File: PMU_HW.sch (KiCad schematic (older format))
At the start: 9 parts, among them J1 Conn_01x08_Male, J2 Conn_01x08_Male, J3 Conn_01x02_Female, U2 ADS8681IPWR

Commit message: lul
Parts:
- U2: symbol Analog_ADC:ADS8681IPWR -> Analog_ADC:ADS8681IRPWR
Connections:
- wire segments 22 -> 35
- no-connect marks 0 -> 3
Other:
- moved on the sheet: C1, C2, C3, C4, C5, J1, J2, J3

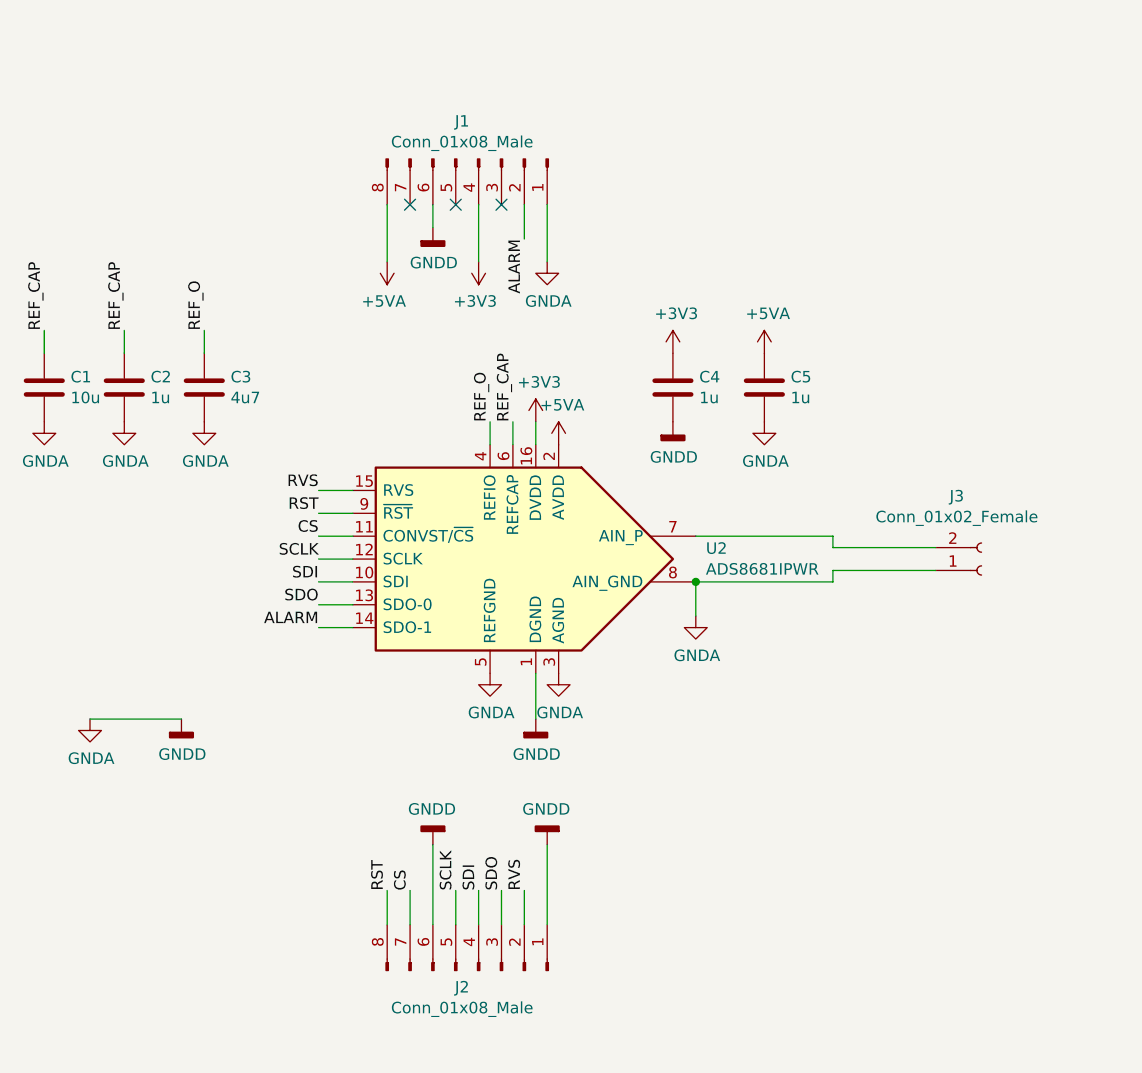
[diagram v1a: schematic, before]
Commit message: finished
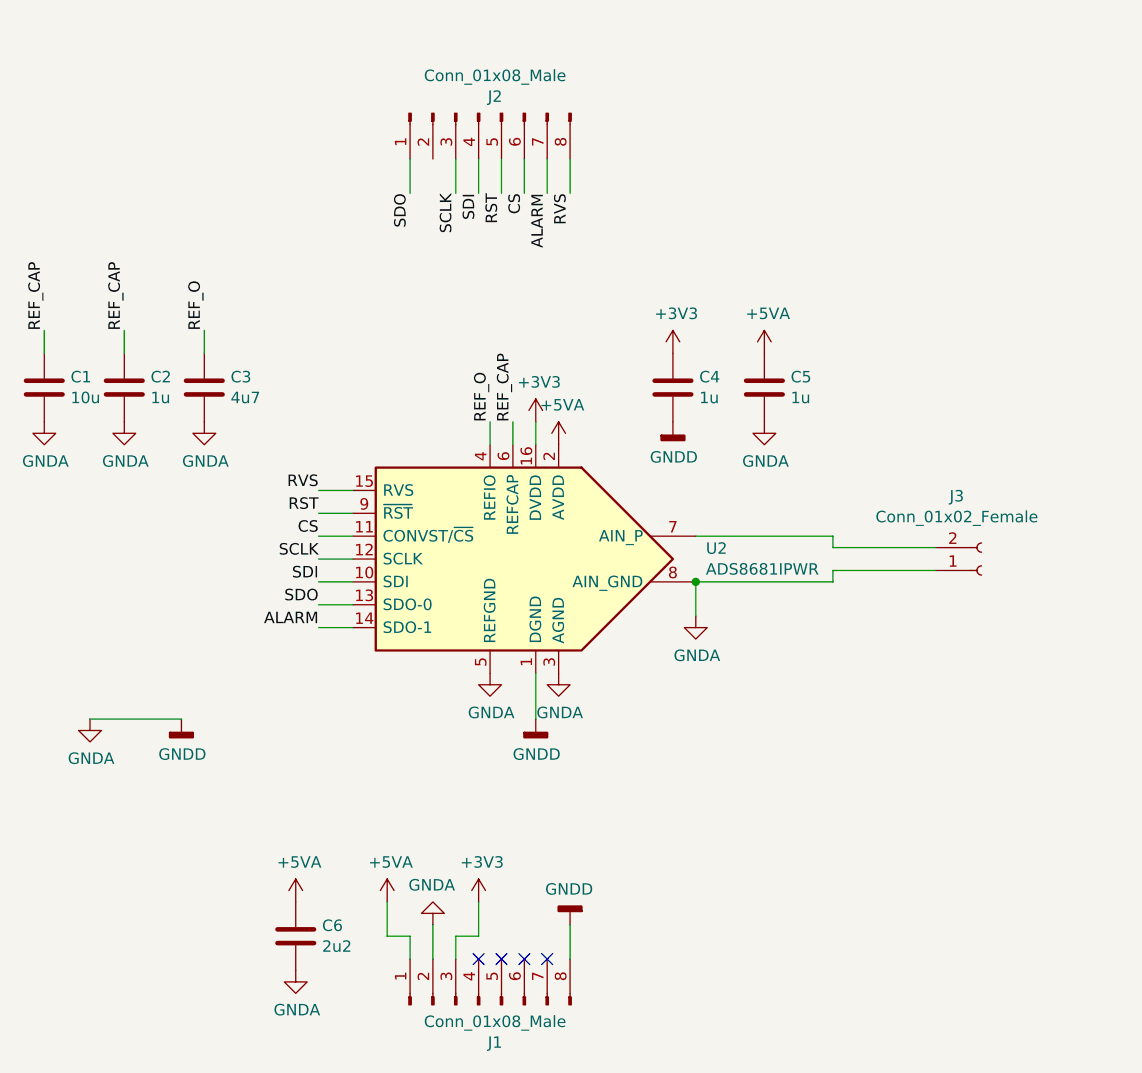
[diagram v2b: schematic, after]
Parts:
- added C6: 2u2, Capacitor_SMD:C_0603_1608Metric_Pad1.08x0.95mm_HandSolder, symbol Device:C
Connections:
- net +3V3: now also J1.3 (Pin_3); no longer J1.4 (Pin_4)
- net +5VA: now also J1.1 (Pin_1), C6.1; no longer J1.8 (Pin_8)
- net ALARM: now also J2.7 (Pin_7); no longer J1.2 (Pin_2)
- net CS: now also J2.6 (Pin_6); no longer J2.7 (Pin_7)
- net GNDA: now also J1.2 (Pin_2), J1.8 (Pin_8), C6.2; no longer J1.1 (Pin_1), J1.6 (Pin_6), J2.1 (Pin_1), J2.6 (Pin_6)
- net RST: now also J2.5 (Pin_5); no longer J2.8 (Pin_8)
- net RVS: now also J2.8 (Pin_8); no longer J2.2 (Pin_2)
- net SCLK: now also J2.3 (Pin_3); no longer J2.5 (Pin_5)
- net SDO: now also J2.1 (Pin_1); no longer J2.3 (Pin_3)
- no-connect marks 3 -> 4
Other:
- moved on the sheet: J1, J2
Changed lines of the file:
@@
 L Connector:Conn_01x08_Male J2
 U 1 1 61E7119A
-P 4950 6300
-F 0 "J2" V 4877 6228 50  0000 C CNN
-F 1 "Conn_01x08_Male" V 4786 6228 50  0000 C CNN
-F 2 "Connector_PinHeader_2.54mm:PinHeader_1x08_P2.54mm_Vertical" H 4950 6300 50  0001 C CNN
-F 3 "~" H 4950 6300 50  0001 C CNN
-	1    4950 6300
-	0    1    -1   0
+P 4950 2550
+F 0 "J2" V 4877 2478 50  0000 C CNN
+F 1 "Conn_01x08_Male" V 4786 2478 50  0000 C CNN
+F 2 "Connector_PinHeader_2.54mm:PinHeader_1x08_P2.54mm_Vertical" H 4950 2550 50  0001 C CNN
+F 3 "~" H 4950 2550 50  0001 C CNN
+	1    4950 2550
+	0    -1   1    0
 $EndComp
 $Comp
@@
 	3250 5200 3650 5200
 Wire Wire Line
-	4550 3200 4550 2950
-Wire Wire Line
-	4750 3050 4750 2950
-Wire Wire Line
-	4950 3200 4950 2950
-Wire Wire Line
-	5250 3200 5250 2950
-$Comp
-L power:+5VA #PWR0116
-U 1 1 61E5BE24
-P 4550 3200
-F 0 "#PWR0116" H 4550 3050 50  0001 C CNN
-F 1 "+5VA" H 4565 3373 50  0000 C CNN
-F 2 "" H 4550 3200 50  0001 C CNN
-F 3 "" H 4550 3200 50  0001 C CNN
-	1    4550 3200
-	-1   0    0    1
-$EndComp
-$Comp
-L power:+3V3 #PWR0117
-U 1 1 61E5D7E7
-P 4950 3200
-F 0 "#PWR0117" H 4950 3050 50  0001 C CNN
-F 1 "+3V3" H 4965 3373 50  0000 C CNN
-F 2 "" H 4950 3200 50  0001 C CNN
-F 3 "" H 4950 3200 50  0001 C CNN
-	1    4950 3200
-	-1   0    0    1
-$EndComp
+	4550 6000 4550 6150
 $Comp
 L Connector:Conn_01x08_Male J1
 U 1 1 61E72333
-P 4950 2750
-F 0 "J1" V 4785 2678 50  0000 C CNN
-F 1 "Conn_01x08_Male" V 4876 2678 50  0000 C CNN
-F 2 "Connector_PinHeader_2.54mm:PinHeader_1x08_P2.54mm_Vertical" H 4950 2750 50  0001 C CNN
-F 3 "~" H 4950 2750 50  0001 C CNN
-	1    4950 2750
-	0    1    1    0
-$EndComp
-NoConn ~ 4850 2950
-NoConn ~ 4650 2950
-$Comp
-L power:GNDA #PWR0118
-U 1 1 61E5F744
-P 5250 3200
-F 0 "#PWR0118" H 5250 2950 50  0001 C CNN
-F 1 "GNDA" H 5255 3027 50  0000 C CNN
-F 2 "" H 5250 3200 50  0001 C CNN
-F 3 "" H 5250 3200 50  0001 C CNN
-	1    5250 3200
-	1    0    0    -1
-$EndComp
-$Comp
-L power:GNDD #PWR0119
-U 1 1 61E5FCEF
-P 4750 3050
-F 0 "#PWR0119" H 4750 2800 50  0001 C CNN
-F 1 "GNDD" H 4754 2895 50  0000 C CNN
-F 2 "" H 4750 3050 50  0001 C CNN
-F 3 "" H 4750 3050 50  0001 C CNN
-	1    4750 3050
-	1    0    0    -1
-$EndComp
-NoConn ~ 5050 2950
-$Comp
-L power:GNDD #PWR0120
-U 1 1 61E6084F
-P 4750 5750
-F 0 "#PWR0120" H 4750 5500 50  0001 C CNN
-F 1 "GNDD" H 4754 5595 50  0000 C CNN
-F 2 "" H 4750 5750 50  0001 C CNN
-F 3 "" H 4750 5750 50  0001 C CNN
-	1    4750 5750
-	-1   0    0    1
-$EndComp
-Wire Wire Line
-	4750 6100 4750 5750
-Wire Wire Line
-	5250 5750 5250 6100
-Wire Wire Line
-	5150 5950 5150 6100
-Wire Wire Line
-	5050 5950 5050 6100
-Wire Wire Line
-	4950 5950 4950 6100
-Wire Wire Line
-	4850 5950 4850 6100
-Text Label 4850 5950 1    50   ~ 0
-SCLK
-Text Label 4650 5950 1    50   ~ 0
+P 4950 6450
+F 0 "J1" V 4785 6378 50  0000 C CNN
+F 1 "Conn_01x08_Male" V 4876 6378 50  0000 C CNN
+F 2 "Connector_PinHeader_2.54mm:PinHeader_1x08_P2.54mm_Vertical" H 4950 6450 50  0001 C CNN
+F 3 "~" H 4950 6450 50  0001 C CNN
+	1    4950 6450
+	0    -1   -1   0
+$EndComp
+Wire Wire Line
+	5150 2750 5150 2900
+Wire Wire Line
+	4650 2900 4650 2750
+Wire Wire Line
+	4850 2900 4850 2750
+Wire Wire Line
+	4950 2900 4950 2750
+Wire Wire Line
+	5050 2900 5050 2750
+Text Label 5150 2900 3    50   ~ 0
 CS
-Text Label 5050 5950 1    50   ~ 0
+Text Label 4650 2900 3    50   ~ 0
 SDO
-$Comp
-L power:GNDD #PWR0121
-U 1 1 61E64E09
-P 5250 5750
-F 0 "#PWR0121" H 5250 5500 50  0001 C CNN
-F 1 "GNDD" H 5254 5595 50  0000 C CNN
-F 2 "" H 5250 5750 50  0001 C CNN
-F 3 "" H 5250 5750 50  0001 C CNN
-	1    5250 5750
-	-1   0    0    1
-$EndComp
-Text Label 4950 5950 1    50   ~ 0
+Text Label 4950 2900 3    50   ~ 0
 SDI
 Wire Wire Line
-	4650 5950 4650 6100
-Wire Wire Line
-	4550 5950 4550 6100
-Text Label 5150 3100 3    50   ~ 0
-ALARM
-Text Label 5150 5950 1    50   ~ 0
+	5250 2900 5250 2750
+Text Label 5350 2900 3    50   ~ 0
 RVS
 Wire Wire Line
-	5150 2950 5150 3100
-Text Label 4550 5950 1    50   ~ 0
+	4750 6250 4750 6100
+Text Label 5050 2900 3    50   ~ 0
 RST
 Connection ~ 5900 4600
+Text Label 4850 2900 3    50   ~ 0
+SCLK
+Wire Wire Line
+	5350 2750 5350 2900
+$Comp
+L power:+5VA #PWR0116
+U 1 1 61E74B7E
+P 4550 6000
+F 0 "#PWR0116" H 4550 5850 50  0001 C CNN
+F 1 "+5VA" H 4565 6173 50  0000 C CNN
+F 2 "" H 4550 6000 50  0001 C CNN
+F 3 "" H 4550 6000 50  0001 C CNN
+	1    4550 6000
+	1    0    0    -1
+$EndComp
+$Comp
+L power:+3V3 #PWR0117
+U 1 1 61E74F0A
+P 4950 6000
+F 0 "#PWR0117" H 4950 5850 50  0001 C CNN
+F 1 "+3V3" H 4965 6173 50  0000 C CNN
+F 2 "" H 4950 6000 50  0001 C CNN
+F 3 "" H 4950 6000 50  0001 C CNN
+	1    4950 6000
+	1    0    0    -1
+$EndComp
+Wire Wire Line
+	4550 6150 4650 6150
+Wire Wire Line
+	4650 6150 4650 6250
+Wire Wire Line
+	4850 6250 4850 6150
+Wire Wire Line
+	4850 6150 4950 6150
+Wire Wire Line
+	4950 6150 4950 6000
+$Comp
+L power:GNDA #PWR0118
+U 1 1 61E780C9
+P 4750 6100
+F 0 "#PWR0118" H 4750 5850 50  0001 C CNN
+F 1 "GNDA" H 4755 5927 50  0000 C CNN
+F 2 "" H 4750 6100 50  0001 C CNN
+F 3 "" H 4750 6100 50  0001 C CNN
+	1    4750 6100
+	-1   0    0    1
+$EndComp
+$Comp
+L power:GNDD #PWR0119
+U 1 1 61E78930
+P 5350 6100
+F 0 "#PWR0119" H 5350 5850 50  0001 C CNN
+F 1 "GNDD" H 5354 5945 50  0000 C CNN
+F 2 "" H 5350 6100 50  0001 C CNN
+F 3 "" H 5350 6100 50  0001 C CNN
+	1    5350 6100
+	-1   0    0    1
+$EndComp
+Wire Wire Line
+	5350 6250 5350 6100
+NoConn ~ 4950 6250
+NoConn ~ 5050 6250
+NoConn ~ 5150 6250
+NoConn ~ 5250 6250
+Text Label 5250 2900 3    50   ~ 0
+ALARM
+$Comp
+L Device:C C6
+U 1 1 61E6A197
+P 4150 6150
+F 0 "C6" H 4265 6196 50  0000 L CNN
+F 1 "2u2" H 4265 6105 50  0000 L CNN
+F 2 "Capacitor_SMD:C_0603_1608Metric_Pad1.08x0.95mm_HandSolder" H 4188 6000 50  0001 C CNN
+F 3 "~" H 4150 6150 50  0001 C CNN
+	1    4150 6150
+	1    0    0    -1
+$EndComp
+$Comp
+L power:+5VA #PWR?
+U 1 1 61E6A51A
+P 4150 6000
+F 0 "#PWR?" H 4150 5850 50  0001 C CNN
+F 1 "+5VA" H 4165 6173 50  0000 C CNN
+F 2 "" H 4150 6000 50  0001 C CNN
+F 3 "" H 4150 6000 50  0001 C CNN
+	1    4150 6000
+	1    0    0    -1
+$EndComp
+$Comp
+L power:GNDA #PWR?
+U 1 1 61E6A807
+P 4150 6300
+F 0 "#PWR?" H 4150 6050 50  0001 C CNN
+F 1 "GNDA" H 4155 6127 50  0000 C CNN
+F 2 "" H 4150 6300 50  0001 C CNN
+F 3 "" H 4150 6300 50  0001 C CNN
+	1    4150 6300
+	1    0    0    -1
+$EndComp
 $EndSCHEMATC
